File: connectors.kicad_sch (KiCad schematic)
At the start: 6 parts, among them J1 Conn_01x04_Pin, J10 Conn_01x06_Pin, J13 Conn_02x04_Counter_Clockwise, J14 Conn_02x04_Counter_Clockwise, J2 Conn_01x04_Pin, J9 Conn_01x04_Pin

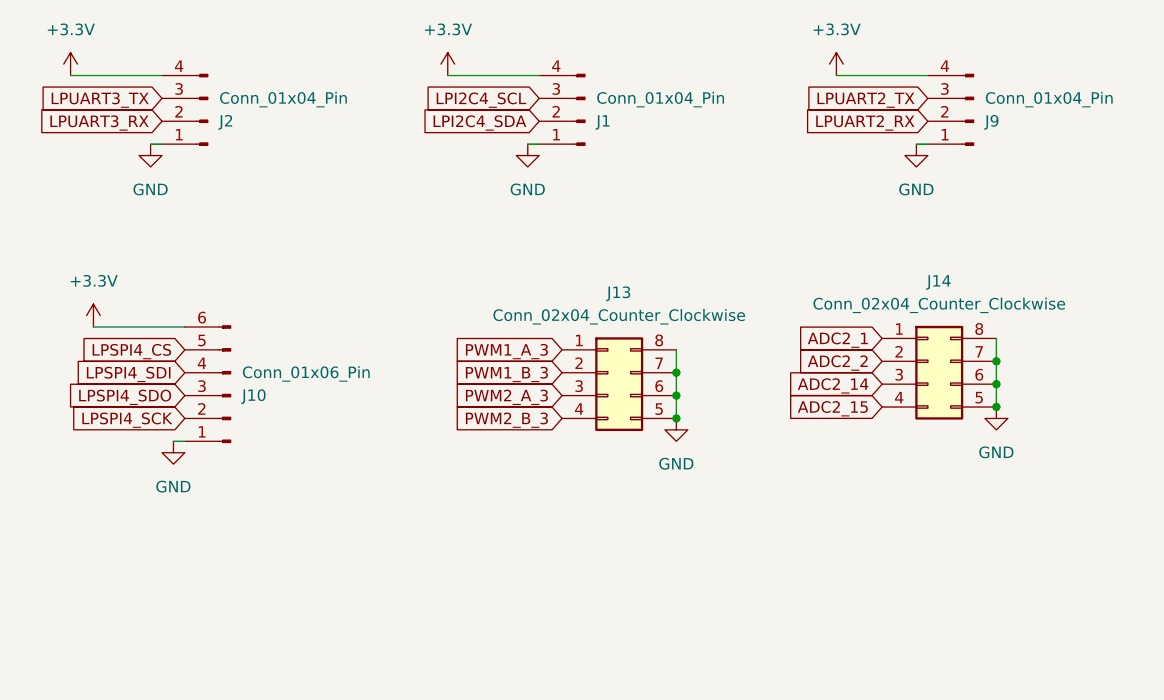
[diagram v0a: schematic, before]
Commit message: v0.2
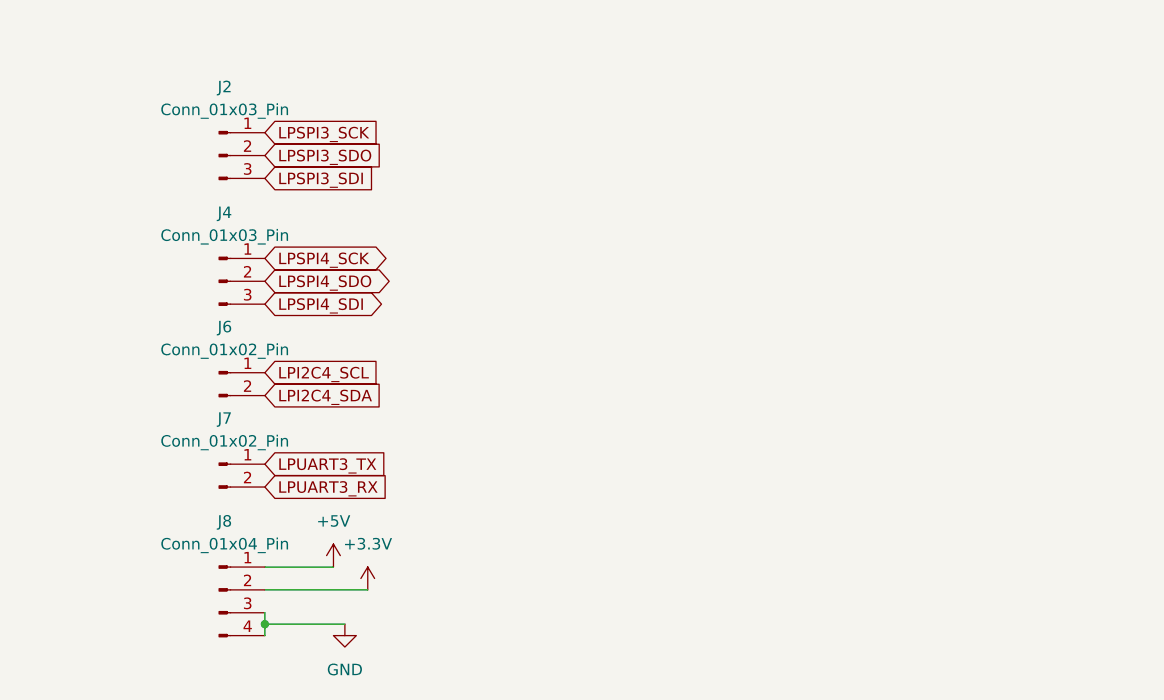
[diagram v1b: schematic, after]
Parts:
- removed J1, J2, J9: Conn_01x04_Pin, Connector_PinHeader_2.00mm:PinHeader_1x04_P2.00mm_Vertical, symbol Connector:Conn_01x04_Pin
- removed J10: Conn_01x06_Pin, Connector_PinHeader_2.00mm:PinHeader_1x06_P2.00mm_Vertical, symbol Connector:Conn_01x06_Pin
- removed J13, J14: Conn_02x04_Counter_Clockwise, Connector_PinHeader_2.00mm:PinHeader_2x04_P2.00mm_Vertical, symbol Connector_Generic:Conn_02x04_Counter_Clockwise
- added J2, J4: Conn_01x03_Pin, symbol Connector:Conn_01x03_Pin
- added J6, J7: Conn_01x02_Pin, symbol Connector:Conn_01x02_Pin
- added J8: Conn_01x04_Pin, symbol Connector:Conn_01x04_Pin
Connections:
- net +3.3V: now also J8.2 (Pin_2)
- net GND: now also J8.3 (Pin_3), J8.4 (Pin_4)
- net LPI2C4_SCL: now also J6.1 (Pin_1)
- net LPI2C4_SDA: now also J6.2 (Pin_2)
- net LPSPI4_SCK: now also J4.1 (Pin_1)
- net LPSPI4_SDI: now also J4.3 (Pin_3)
- net LPSPI4_SDO: now also J4.2 (Pin_2)
- net LPUART3_RX: now also J7.2 (Pin_2)
- net LPUART3_TX: now also J7.1 (Pin_1)
- new net +5V: J8.1 (Pin_1)
- new net LPSPI3_SCK: J2.1 (Pin_1)
- new net LPSPI3_SDI: J2.3 (Pin_3)
- new net LPSPI3_SDO: J2.2 (Pin_2)
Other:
- title: RT1050 DevBoard for Project Horizon -> Payload Board for Pleiades Atlas

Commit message: started layout
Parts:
- J2, J4: footprint (none) -> Connector_PinHeader_1.00mm:PinHeader_1x03_P1.00mm_Vertical
- J6, J7: footprint (none) -> Connector_PinHeader_1.00mm:PinHeader_1x02_P1.00mm_Vertical
- J8: footprint (none) -> Connector_PinHeader_1.00mm:PinHeader_1x04_P1.00mm_Vertical
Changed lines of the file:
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@@
 			)
 		)
-		(property "Footprint" ""
+		(property "Footprint" "Connector_PinHeader_1.00mm:PinHeader_1x02_P1.00mm_Vertical"
 			(at 35.56 55.88 0)
 			(effects
@@
 			)
 		)
-		(property "Footprint" ""
+		(property "Footprint" "Connector_PinHeader_1.00mm:PinHeader_1x04_P1.00mm_Vertical"
 			(at 35.56 80.01 0)
 			(effects
@@
 			)
 		)
-		(property "Footprint" ""
+		(property "Footprint" "Connector_PinHeader_1.00mm:PinHeader_1x02_P1.00mm_Vertical"
 			(at 35.56 66.04 0)
 			(effects
@@
 			)
 		)
-		(property "Footprint" ""
+		(property "Footprint" "Connector_PinHeader_1.00mm:PinHeader_1x03_P1.00mm_Vertical"
 			(at 35.56 45.72 0)
 			(effects
@@
 			)
 		)
-		(property "Footprint" ""
+		(property "Footprint" "Connector_PinHeader_1.00mm:PinHeader_1x03_P1.00mm_Vertical"
 			(at 35.56 31.75 0)
 			(effects

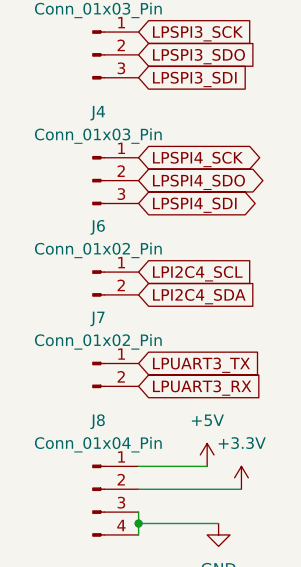
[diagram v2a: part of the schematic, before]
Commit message: finished layout of v0.2!
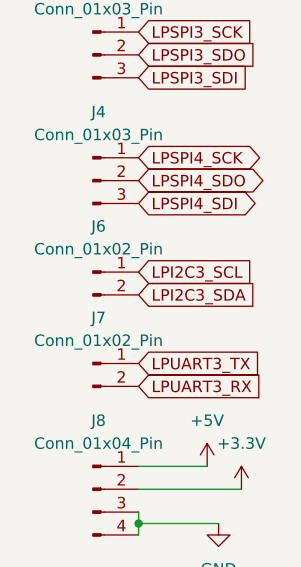
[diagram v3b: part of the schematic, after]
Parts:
- J2, J4: footprint Connector_PinHeader_1.00mm:PinHeader_1x03_P1.00mm_Vertical -> Connector_PinHeader_2.54mm:PinHeader_1x03_P2.54mm_Vertical
- J6, J7: footprint Connector_PinHeader_1.00mm:PinHeader_1x02_P1.00mm_Vertical -> Connector_PinHeader_2.54mm:PinHeader_1x02_P2.54mm_Vertical
- J8: footprint Connector_PinHeader_1.00mm:PinHeader_1x04_P1.00mm_Vertical -> Connector_PinHeader_2.54mm:PinHeader_1x04_P2.54mm_Vertical
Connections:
- net LPI2C4_SCL renamed LPI2C3_SCL
- net LPI2C4_SDA renamed LPI2C3_SDA
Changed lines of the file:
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@@
 		)
 	)
-	(global_label "LPI2C4_SCL"
+	(global_label "LPI2C3_SCL"
 		(shape input)
 		(at 40.64 55.88 0)
@@
 		)
 	)
-	(global_label "LPI2C4_SDA"
+	(global_label "LPUART3_TX"
 		(shape input)
-		(at 40.64 58.42 0)
+		(at 40.64 66.04 0)
 		(fields_autoplaced yes)
 		(effects
@@
 		)
 		(property "Intersheetrefs" "${INTERSHEET_REFS}"
-			(at 54.7528 58.42 0)
+			(at 54.9342 66.04 0)
 			(effects
 				(font
@@
 		)
 	)
-	(global_label "LPUART3_TX"
+	(global_label "LPSPI3_SDI"
 		(shape input)
-		(at 40.64 66.04 0)
+		(at 40.64 34.29 0)
 		(fields_autoplaced yes)
 		(effects
@@
 		)
 		(property "Intersheetrefs" "${INTERSHEET_REFS}"
-			(at 54.9342 66.04 0)
+			(at 54.269 34.29 0)
 			(effects
 				(font
@@
 		)
 	)
-	(global_label "LPSPI3_SDI"
+	(global_label "LPI2C3_SDA"
 		(shape input)
-		(at 40.64 34.29 0)
+		(at 40.64 58.42 0)
 		(fields_autoplaced yes)
 		(effects
@@
 		)
 		(property "Intersheetrefs" "${INTERSHEET_REFS}"
-			(at 54.269 34.29 0)
+			(at 54.7528 58.42 0)
 			(effects
 				(font
@@
 			)
 		)
-		(property "Footprint" "Connector_PinHeader_1.00mm:PinHeader_1x02_P1.00mm_Vertical"
+		(property "Footprint" "Connector_PinHeader_2.54mm:PinHeader_1x02_P2.54mm_Vertical"
 			(at 35.56 55.88 0)
 			(effects
@@
 			)
 		)
-		(property "Footprint" "Connector_PinHeader_1.00mm:PinHeader_1x04_P1.00mm_Vertical"
+		(property "Footprint" "Connector_PinHeader_2.54mm:PinHeader_1x04_P2.54mm_Vertical"
 			(at 35.56 80.01 0)
 			(effects
@@
 			)
 		)
-		(property "Footprint" "Connector_PinHeader_1.00mm:PinHeader_1x02_P1.00mm_Vertical"
+		(property "Footprint" "Connector_PinHeader_2.54mm:PinHeader_1x02_P2.54mm_Vertical"
 			(at 35.56 66.04 0)
 			(effects
@@
 			)
 		)
-		(property "Footprint" "Connector_PinHeader_1.00mm:PinHeader_1x03_P1.00mm_Vertical"
+		(property "Footprint" "Connector_PinHeader_2.54mm:PinHeader_1x03_P2.54mm_Vertical"
 			(at 35.56 45.72 0)
 			(effects
@@
 			)
 		)
-		(property "Footprint" "Connector_PinHeader_1.00mm:PinHeader_1x03_P1.00mm_Vertical"
+		(property "Footprint" "Connector_PinHeader_2.54mm:PinHeader_1x03_P2.54mm_Vertical"
 			(at 35.56 31.75 0)
 			(effects
